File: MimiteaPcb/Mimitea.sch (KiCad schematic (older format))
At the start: 26 parts

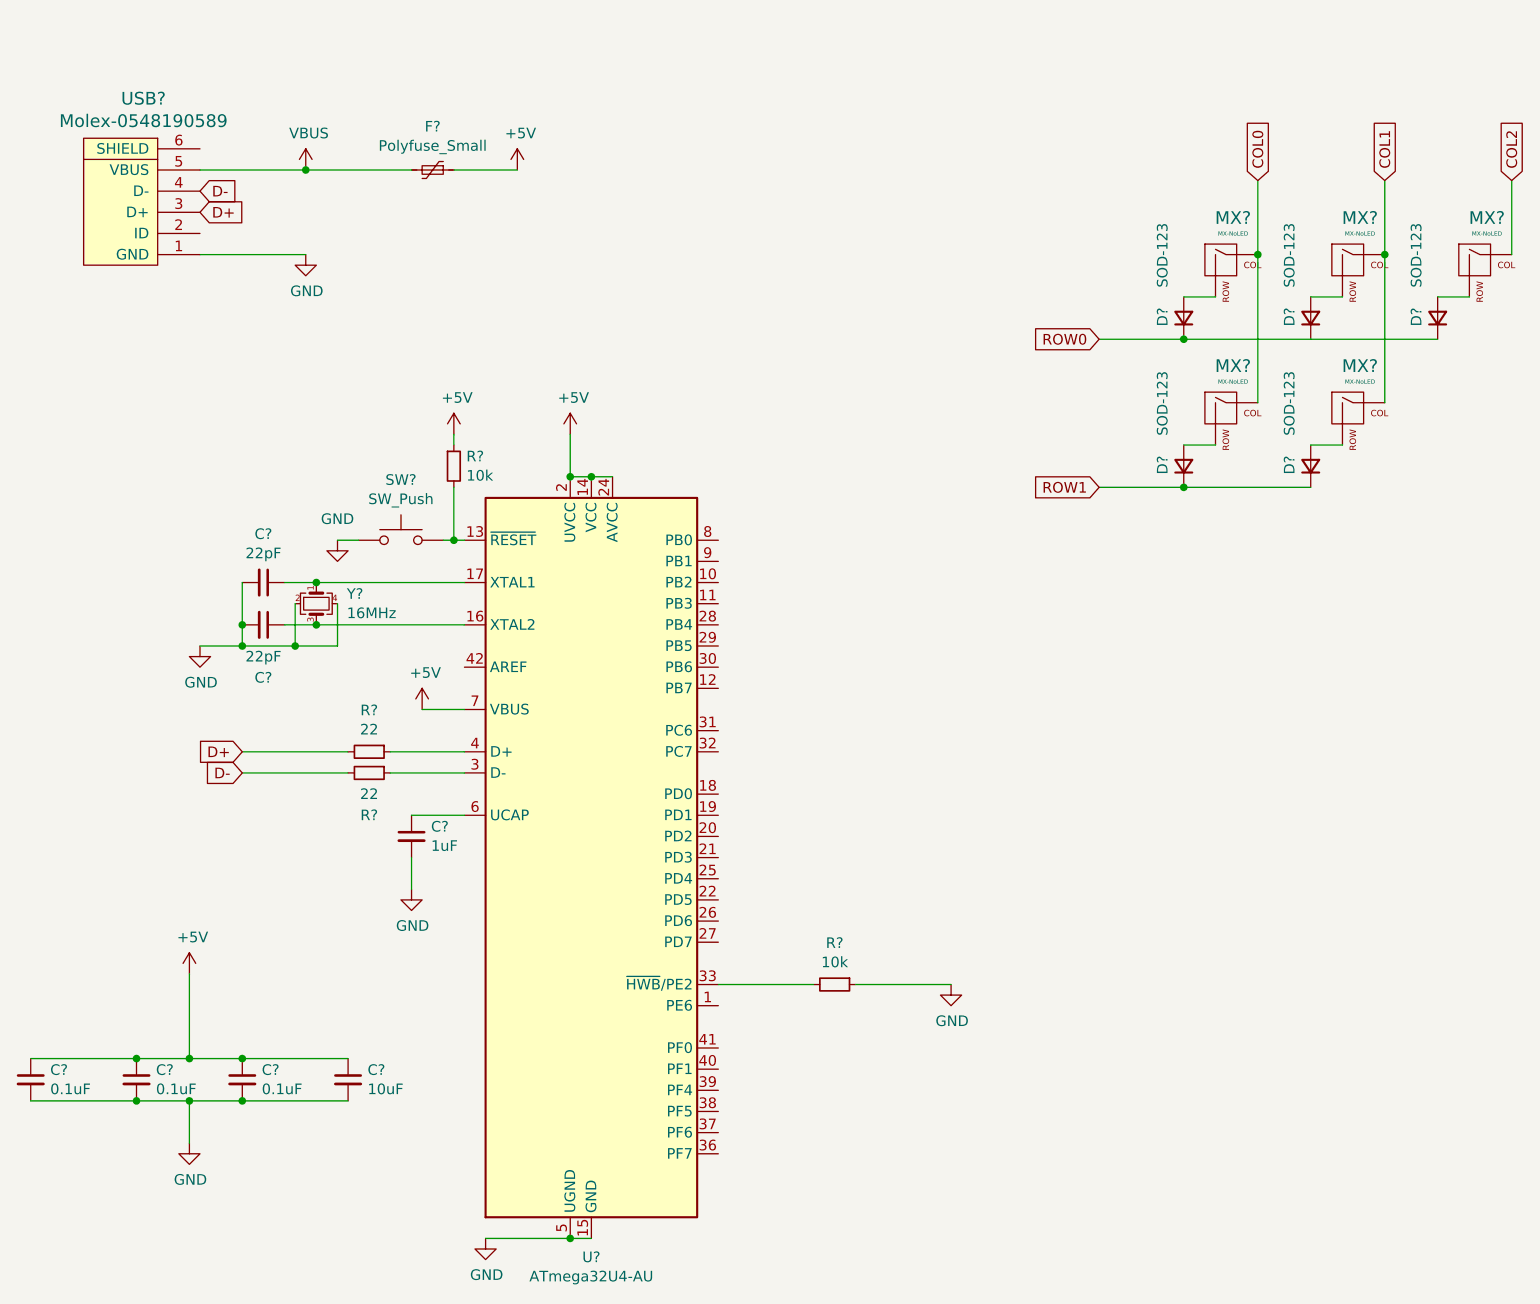
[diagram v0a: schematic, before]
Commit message: Revert "Removed submodule"
This reverts commit a926e21116d6c2bed23dd5c12b6762beb5b98602.
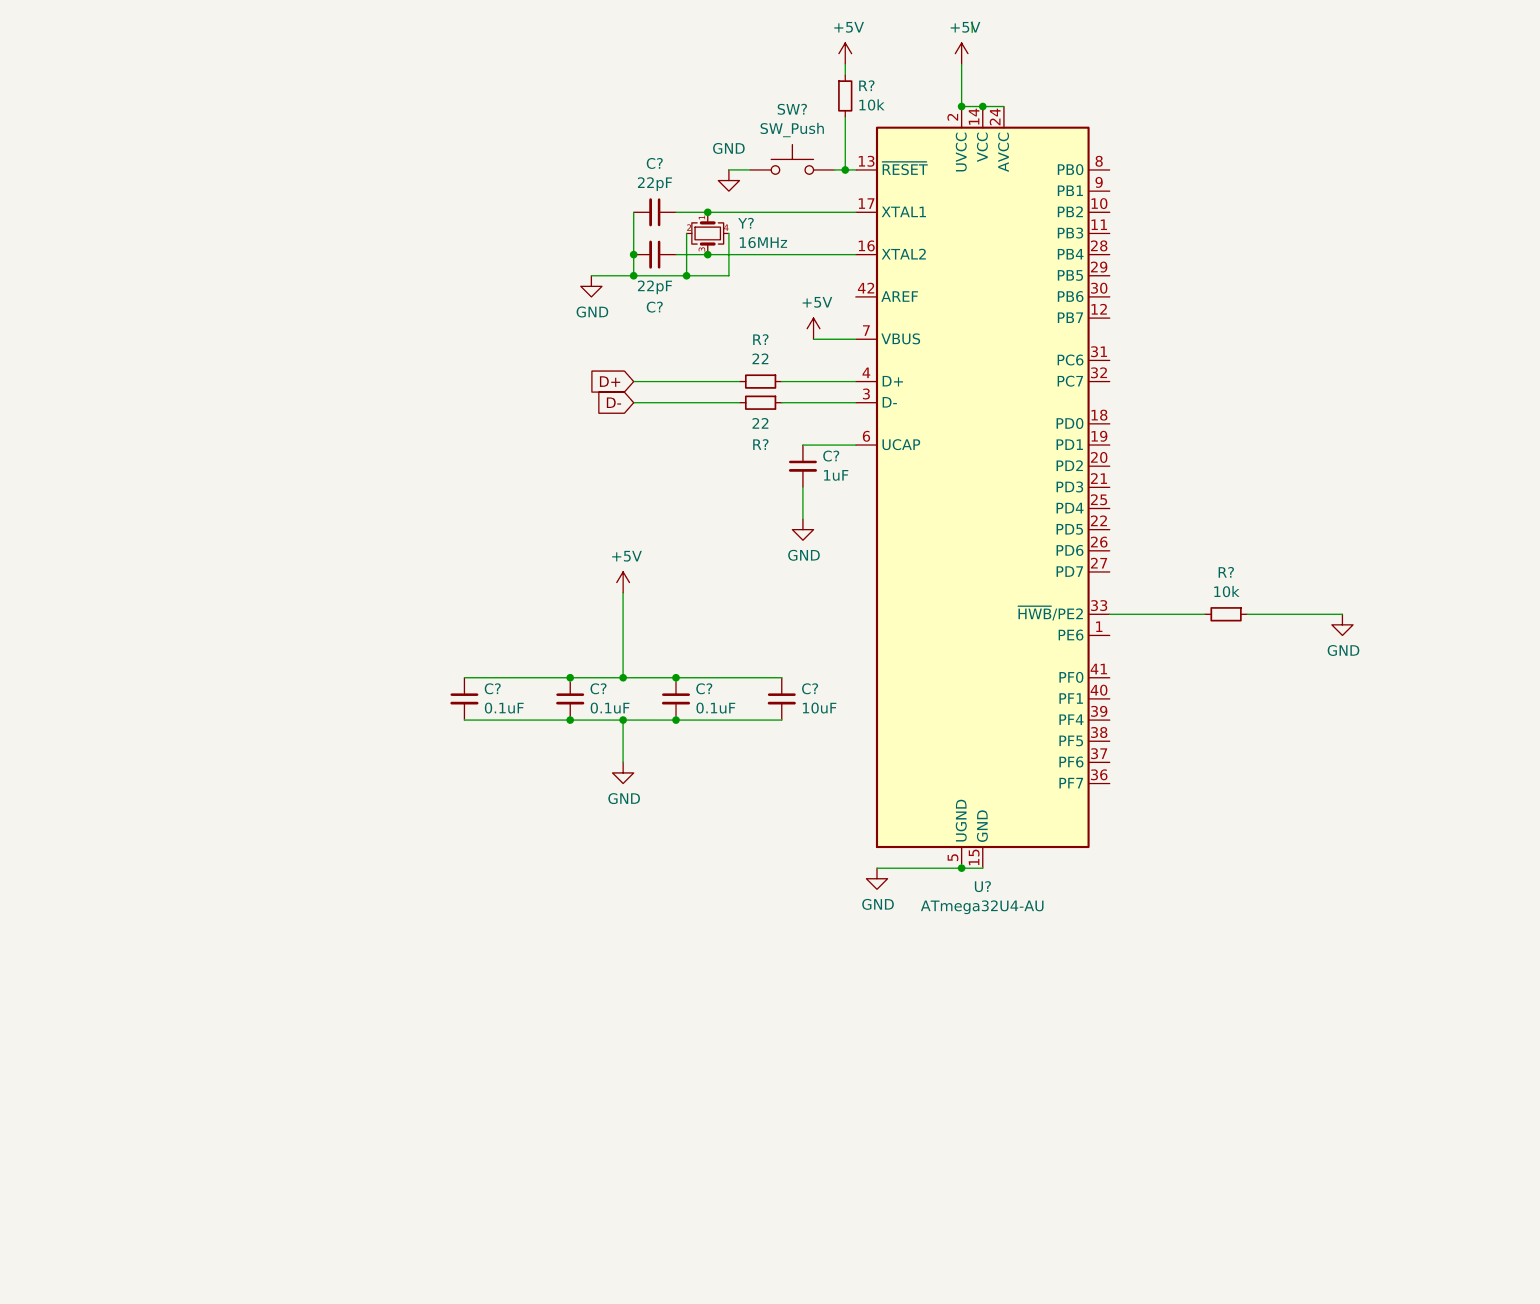
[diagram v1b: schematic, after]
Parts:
- removed D? (x5): SOD-123, symbol Device:D_Small
- removed F?: Polyfuse_Small, symbol Device:Polyfuse_Small
- removed MX? (x5): MX-NoLED, symbol MX_Alps_Hybrid:MX-NoLED
- removed USB?: Molex-0548190589, symbol random-keyboard-parts:Molex-0548190589
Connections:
- net labels removed: COL0, COL1, COL2, ROW0, ROW1, VBUS
- wire segments 59 -> 41
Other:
- moved on the sheet: C?, R?, SW?, U?, Y?
